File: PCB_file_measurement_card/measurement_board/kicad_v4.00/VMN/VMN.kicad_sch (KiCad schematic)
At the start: 43 parts, among them J1 A/B, J2 Screw_Terminal_VMN, J3 Alim DPH5005, J4 Raspberry_Pi_2_3, K1 AQY211EH, K2 AQY211EH, K3 AQY211EH, K4 AQY211EH, U1 INA128, U2 MCP23008-xP, U3 LM358, U4 INA282, U5 1085-Adress=0X49, U6 1085-Adress=0X48, U7 ISO1540

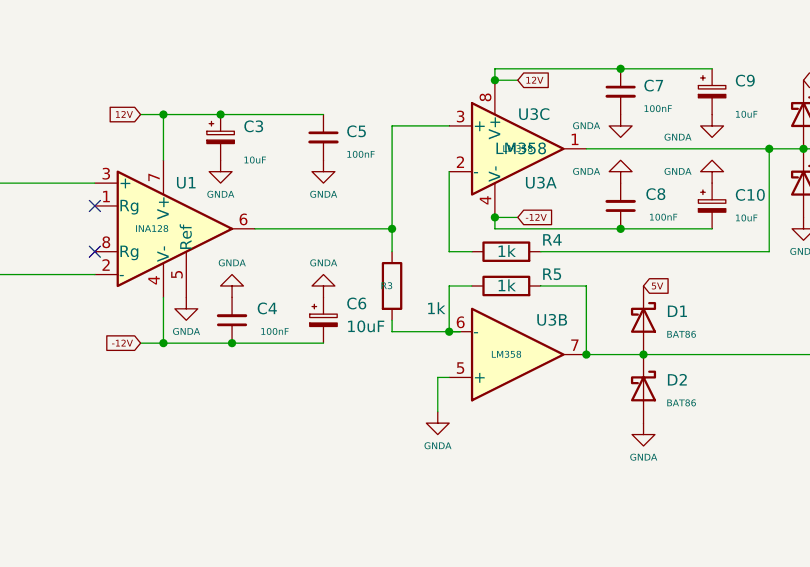
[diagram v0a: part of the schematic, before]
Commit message: Adds a first version of the PCB to be checked...
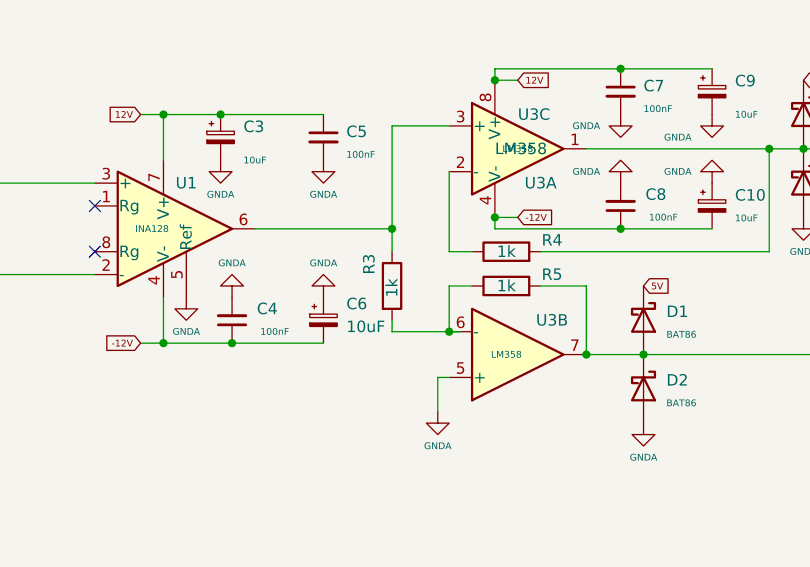
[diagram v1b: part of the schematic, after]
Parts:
- R6: footprint Resistor_THT:R_Axial_DIN0411_L9.9mm_D3.6mm_P15.24mm_Horizontal -> Resistor_THT:R_Axial_DIN0414_L11.9mm_D4.5mm_P20.32mm_Horizontal
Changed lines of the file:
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@@
       (effects (font (size 1.27 1.27)) (justify left))
     )
-    (property "Footprint" "Resistor_THT:R_Axial_DIN0411_L9.9mm_D3.6mm_P15.24mm_Horizontal" (id 2) (at 107.442 133.35 90)
+    (property "Footprint" "Resistor_THT:R_Axial_DIN0414_L11.9mm_D4.5mm_P20.32mm_Horizontal" (id 2) (at 107.442 133.35 90)
       (effects (font (size 1.27 1.27)) hide)
     )
@@
   (symbol (lib_id "Device:R") (at 86.36 80.01 0) (unit 1)
     (in_bom yes) (on_board yes)
-    (property "Reference" "R3" (id 0) (at 85.09 80.01 0)
-      (effects (font (size 0.75 0.75)) (justify left))
-    )
-    (property "Value" "1k" (id 1) (at 90.17 82.5499 0)
+    (property "Reference" "R3" (id 0) (at 83.82 78.74 90)
+      (effects (font (size 1.27 1.27)) (justify left))
+    )
+    (property "Value" "1k" (id 1) (at 86.36 81.28 90)
       (effects (font (size 1.27 1.27)) (justify left))
     )
@@
     )
     (path "/4aa539a9-6f3d-4fc3-b2d6-8348016bf7c3"
-      (reference "R6") (unit 1) (value "2") (footprint "Resistor_THT:R_Axial_DIN0411_L9.9mm_D3.6mm_P15.24mm_Horizontal")
+      (reference "R6") (unit 1) (value "2") (footprint "Resistor_THT:R_Axial_DIN0414_L11.9mm_D4.5mm_P20.32mm_Horizontal")
     )
     (path "/cd253d18-2c33-4027-8d8b-dc6d99e23181"
